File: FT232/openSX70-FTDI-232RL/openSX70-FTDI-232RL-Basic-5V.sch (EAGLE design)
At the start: 13 parts, among them J1 687106183722, U1 FT232RLSSOP

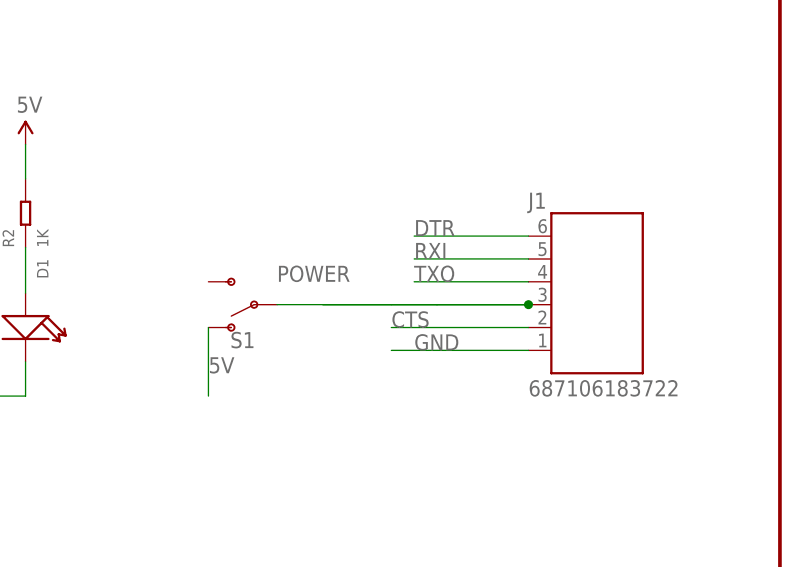
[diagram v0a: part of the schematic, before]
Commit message: Upgrade to 9.1.1 and fixes
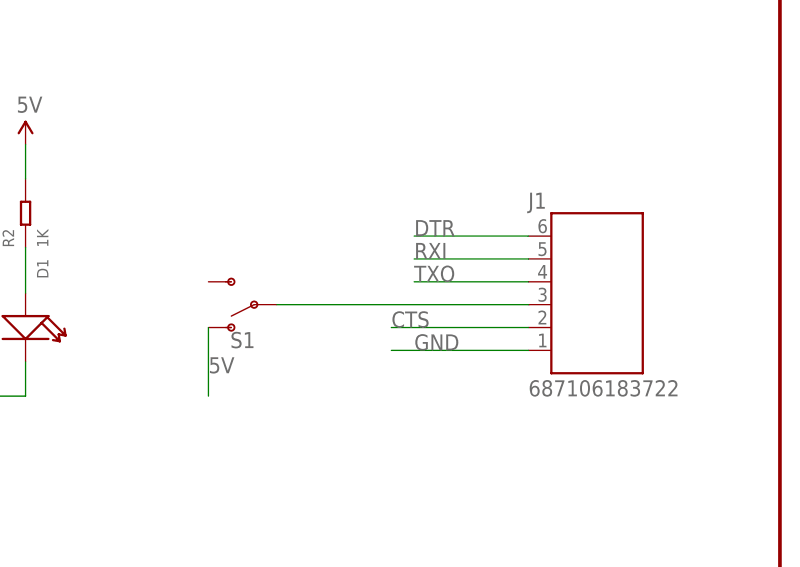
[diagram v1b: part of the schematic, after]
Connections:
- net POWER renamed N$5
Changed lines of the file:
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@@
 <?xml version="1.0" encoding="utf-8"?>
 <!DOCTYPE eagle SYSTEM "eagle.dtd">
-<eagle version="9.0.0">
+<eagle version="9.1.1">
 <drawing>
 <settings>
@@
 </segment>
 </net>
-<net name="POWER" class="0">
-<segment>
-<wire x1="198.12" y1="109.22" x2="205.74" y2="109.22" width="0.1524" layer="91"/>
-<label x="193.04" y="111.76" size="1.778" layer="95"/>
-<pinref part="J1" gate="G$1" pin="4"/>
-<wire x1="210.82" y1="109.22" x2="205.74" y2="109.22" width="0.1524" layer="91"/>
-<wire x1="220.98" y1="109.22" x2="210.82" y2="109.22" width="0.1524" layer="91"/>
-<pinref part="S1" gate="1" pin="P"/>
-<wire x1="193.04" y1="109.22" x2="220.98" y2="109.22" width="0.1524" layer="91"/>
-<junction x="220.98" y="109.22"/>
-</segment>
-</net>
 <net name="5V" class="0">
 <segment>
@@
 </segment>
 </net>
+<net name="N$5" class="0">
+<segment>
+<pinref part="S1" gate="1" pin="P"/>
+<pinref part="J1" gate="G$1" pin="4"/>
+<wire x1="193.04" y1="109.22" x2="220.98" y2="109.22" width="0.1524" layer="91"/>
+</segment>
+</net>
